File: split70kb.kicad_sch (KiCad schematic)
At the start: 2 parts, among them U1 ATMEGA32U4, X1 XTAL_GND

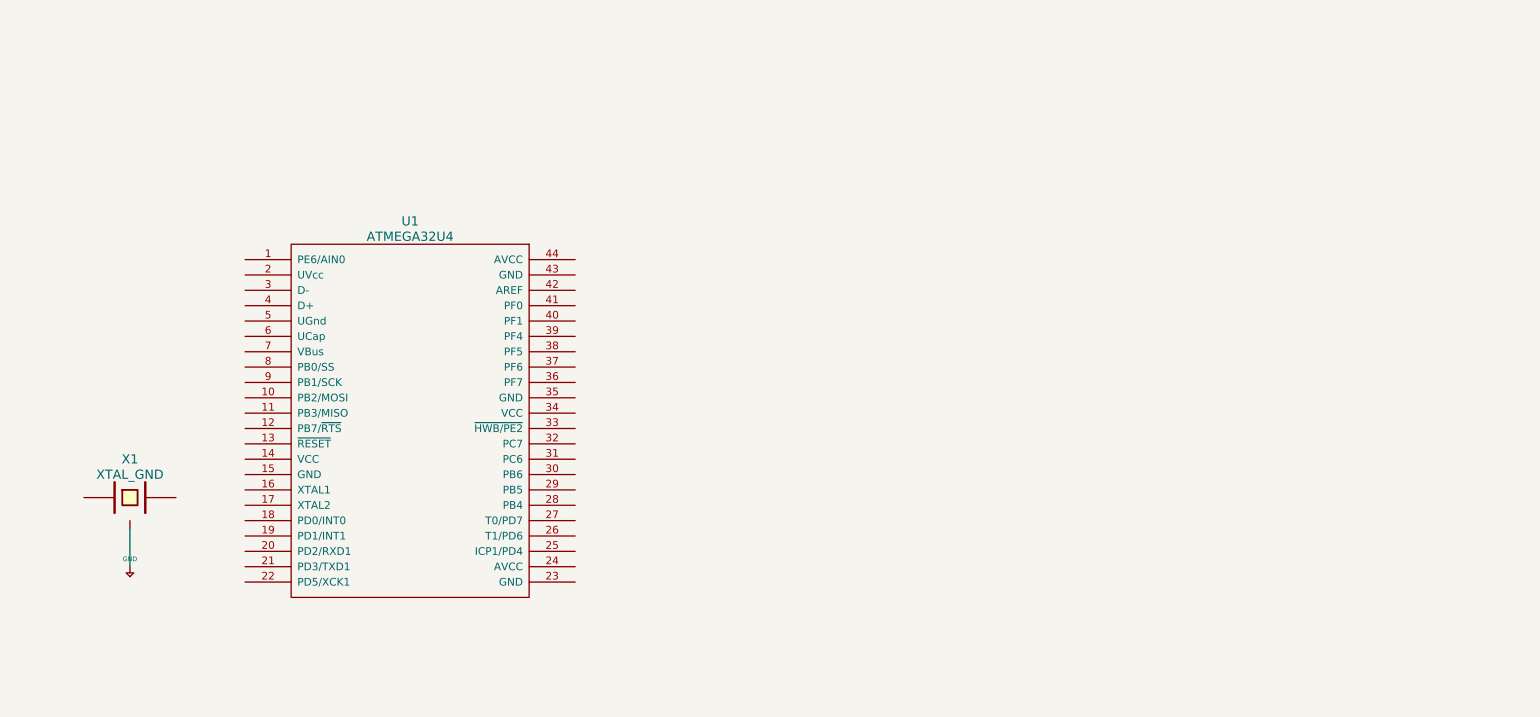
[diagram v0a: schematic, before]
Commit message: finish schematic and pcb layout
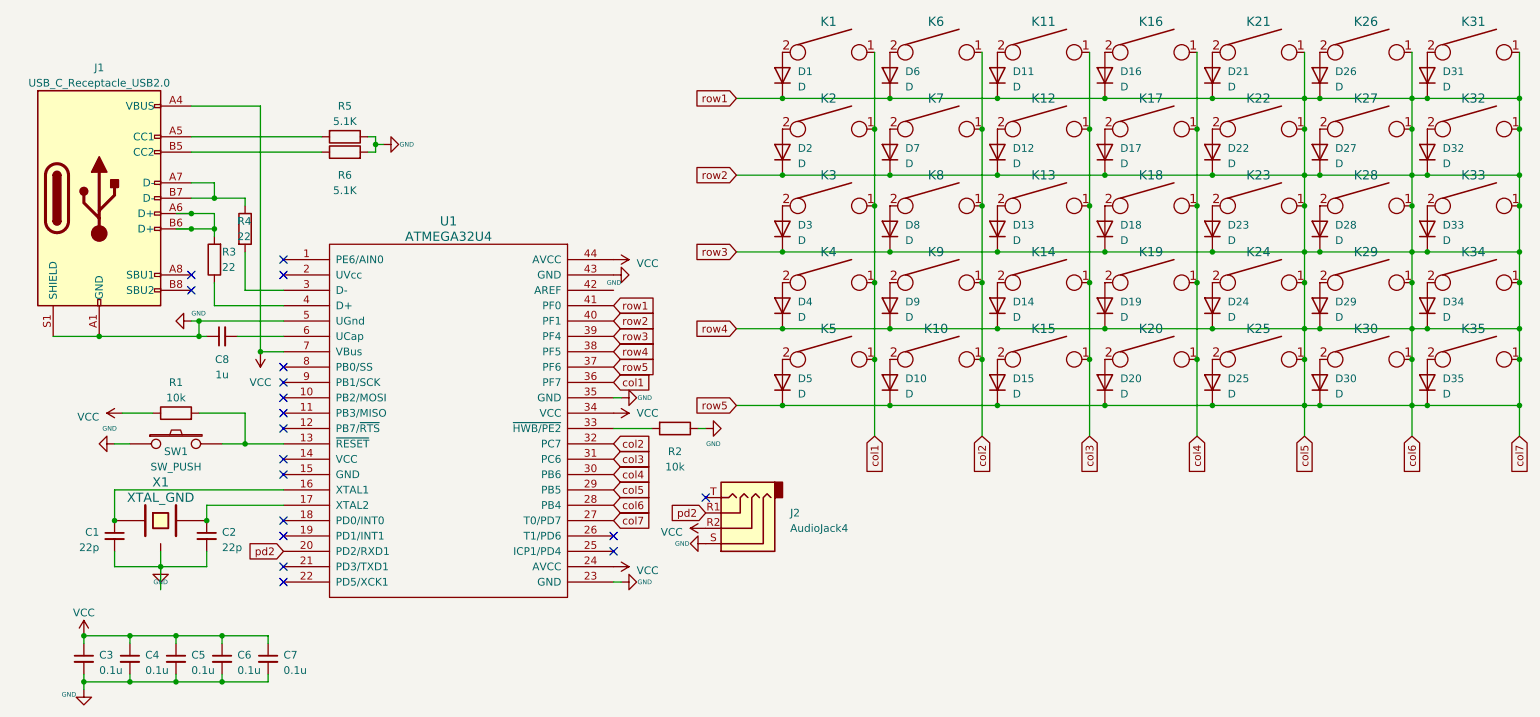
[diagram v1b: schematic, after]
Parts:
- added C1, C2: 22p, Capacitor_SMD:C_0805_2012Metric, symbol Device:C_Small
- added C3, C4, C5, C6, C7: 0.1u, Capacitor_SMD:C_0805_2012Metric, symbol Device:C_Small
- added C8: 1u, Capacitor_SMD:C_0805_2012Metric, symbol Device:C_Small
- added D1, D10, D11, D12, D13, D14, D15, D16, D17, D18, D19, D2, D20, D21, D22, D23, D24, D25, D26, D27, D28, D29, D3, D30, D31, D32, D33, D34, D35, D4, D5, D6, D7, D8, D9: D, keyboard_parts.pretty-master:D_SOD123_axial, symbol Device:D
- added J1: USB_C_Receptacle_USB2.0, Connector_USB:USB_C_Receptacle_Molex_105450-0101, symbol Connector:USB_C_Receptacle_USB2.0
- added J2: AudioJack4, Connector_Audio:Jack_3.5mm_PJ320D_Horizontal, symbol Connector_Audio:AudioJack4
- added K1, K10, K11, K12, K13, K14, K15, K16, K17, K18, K19, K2, K20, K21, K22, K23, K24, K25, K26, K27, K28, K29, K3, K30, K31, K32, K33, K34, K35, K4, K5, K6, K7, K8, K9: KEYSW, keyboard_parts.pretty-master:Mx_Alps_100, symbol keyboard_parts:KEYSW
- added R1, R2: 10k, Resistor_SMD:R_0805_2012Metric, symbol Device:R
- added R3, R4: 22, Resistor_SMD:R_0805_2012Metric, symbol Device:R
- added R5, R6: 5.1K, Resistor_SMD:R_0805_2012Metric, symbol Device:R
- added SW1: SW_PUSH, Button_Switch_SMD:SW_SPST_TL3342, symbol keyboard_parts:SW_PUSH
- U1: footprint (none) -> Package_QFP:TQFP-44_10x10mm_P0.8mm
- X1: footprint (none) -> Crystal:Crystal_SMD_SeikoEpson_FA238-4Pin_3.2x2.5mm
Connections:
- net +5V is gone; now on net GND: X1.3
- net at X1.1: now also U1.16 (XTAL1), C1.1
- net at X1.2: now also U1.17 (XTAL2), C2.1
- net at U1.13 (~{RESET}): now also R1.2, SW1.2
- net pd2: now reaches U1.20 (PD2/RXD1)
- net pd2: now also J2.R1
- net GND: now reaches U1.23 (GND)
- net GND: now also U1.35 (GND), U1.43 (GND), U1.5 (UGnd), C1.2, C2.2, C3.2, C4.2, C5.2, C6.2, C7.2, C8.1, J1.A1 (GND), J1.A12 (GND), J1.B1 (GND), J1.B12 (GND), J1.S1 (SHIELD), J2.S, R2.1, R5.1, R6.2, SW1.1
- net VCC: now reaches U1.24 (AVCC)
- net VCC: now also U1.34 (VCC), U1.44 (AVCC), U1.7 (VBus), C3.1, C4.1, C5.1, C6.1, C7.1, J1.A4 (VBUS), J1.A9 (VBUS), J1.B4 (VBUS), J1.B9 (VBUS), J2.R2, R1.1
- net col5: now reaches U1.27 (T0/PD7)
- net col5: now also U1.28 (PB4), U1.29 (PB5), U1.37 (PF6), U1.38 (PF5), U1.39 (PF4), U1.40 (PF1), U1.41 (PF0), D1.1 (K), D10.1 (K), D11.1 (K), D12.1 (K), D13.1 (K), D14.1 (K), D15.1 (K), D16.1 (K), D17.1 (K), D18.1 (K), D19.1 (K), D2.1 (K), D20.1 (K), D21.1 (K), D22.1 (K), D23.1 (K), D24.1 (K), D25.1 (K), D26.1 (K), D27.1 (K), D28.1 (K), D29.1 (K), D3.1 (K), D30.1 (K), D31.1 (K), D32.1 (K), D33.1 (K), D34.1 (K), D35.1 (K), D4.1 (K), D5.1 (K), D6.1 (K), D7.1 (K), D8.1 (K), D9.1 (K), K21.1, K22.1, K23.1, K24.1, K25.1, K26.1, K27.1, K28.1, K29.1, K30.1, K31.1, K32.1, K33.1, K34.1, K35.1
- net at U1.3 (D-): now also R4.2
- net col4: now reaches U1.30 (PB6)
- net col4: now also K16.1, K17.1, K18.1, K19.1, K20.1
- net col3: now reaches U1.31 (PC6)
- net col3: now also K11.1, K12.1, K13.1, K14.1, K15.1
- net col2: now reaches U1.32 (PC7)
- net col2: now also K10.1, K6.1, K7.1, K8.1, K9.1
- net at U1.33 (~{HWB/PE2}): now also R2.2
- net col1: now reaches U1.36 (PF7)
- net col1: now also K1.1, K2.1, K3.1, K4.1, K5.1
- net at U1.4 (D+): now also R3.1
- net at U1.6 (UCap): now also C8.2
- new net: D5.2 (A), K5.2
- new net: D19.2 (A), K19.2
- new net: D7.2 (A), K7.2
- new net: D17.2 (A), K17.2
- new net: D25.2 (A), K25.2
- new net: D22.2 (A), K22.2
- new net: D35.2 (A), K35.2
- new net: D23.2 (A), K23.2
- new net: D8.2 (A), K8.2
- new net: D21.2 (A), K21.2
- new net: D3.2 (A), K3.2
- new net: D32.2 (A), K32.2
- new net: D29.2 (A), K29.2
- new net: D20.2 (A), K20.2
- new net: D34.2 (A), K34.2
- new net: D16.2 (A), K16.2
- new net: D1.2 (A), K1.2
- new net: D9.2 (A), K9.2
- new net: D27.2 (A), K27.2
- new net: D18.2 (A), K18.2
- new net: D14.2 (A), K14.2
- new net: D10.2 (A), K10.2
- new net: D11.2 (A), K11.2
- new net: D28.2 (A), K28.2
- new net: J1.B5 (CC2), R6.1
- new net: D26.2 (A), K26.2
- new net: D6.2 (A), K6.2
- new net: D33.2 (A), K33.2
- new net: J1.A6 (D+), J1.B6 (D+), R3.2
- new net: D12.2 (A), K12.2
- new net: J1.A5 (CC1), R5.2
- new net: J1.A7 (D-), J1.B7 (D-), R4.1
- new net: D2.2 (A), K2.2
- new net: D31.2 (A), K31.2
- new net: D13.2 (A), K13.2
- new net: D30.2 (A), K30.2
- new net: D15.2 (A), K15.2
- new net: D4.2 (A), K4.2
- new net: D24.2 (A), K24.2
- no-connect marks 0 -> 18
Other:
- moved on the sheet: U1, X1
